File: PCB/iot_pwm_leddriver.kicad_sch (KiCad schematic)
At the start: 17 parts, among them J1 ProgConn-SOICBite, J2 12V PWR, SW1 RESET, SW2 FLASH, U2 ESP-12F

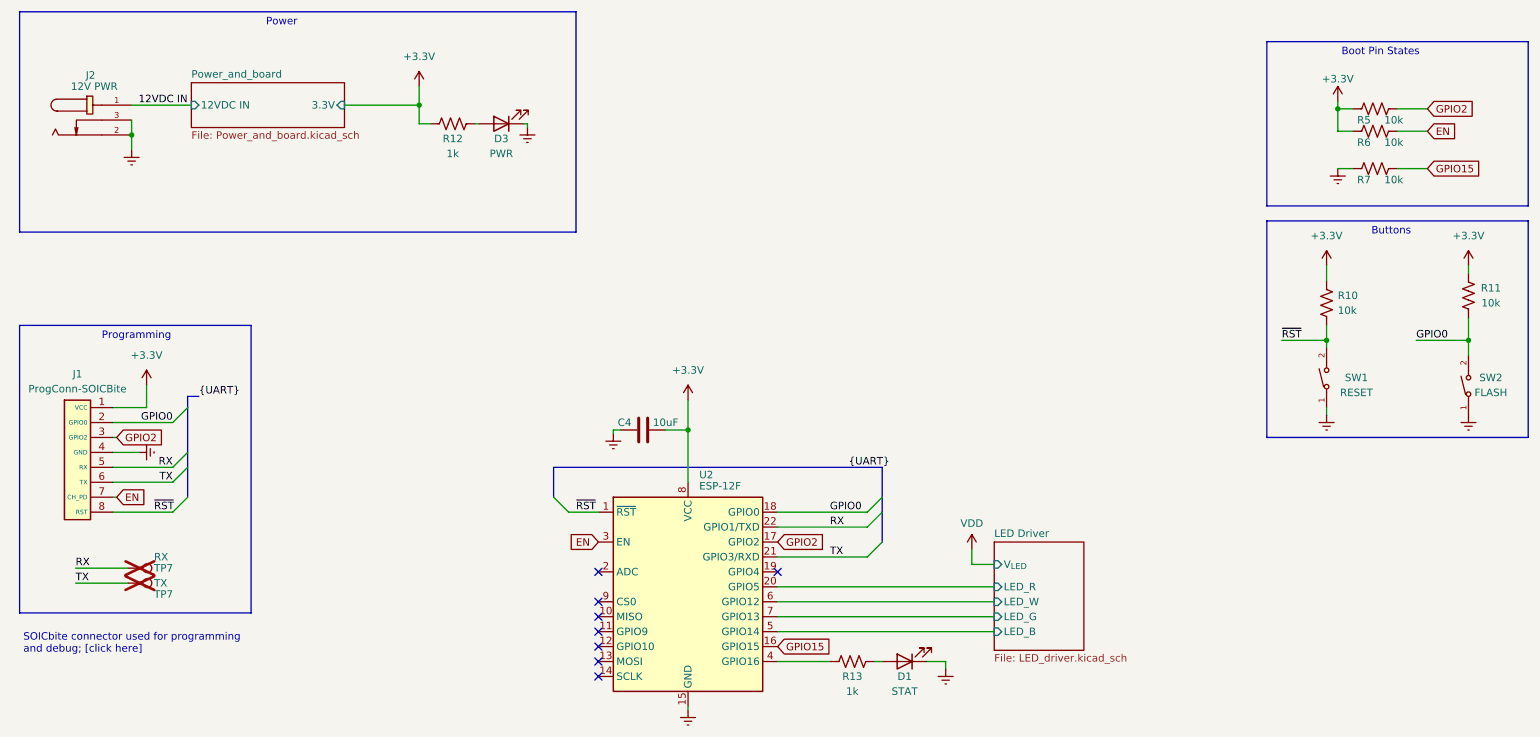
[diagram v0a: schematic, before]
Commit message: schematic and layout cleanup
* plus BOM finalization
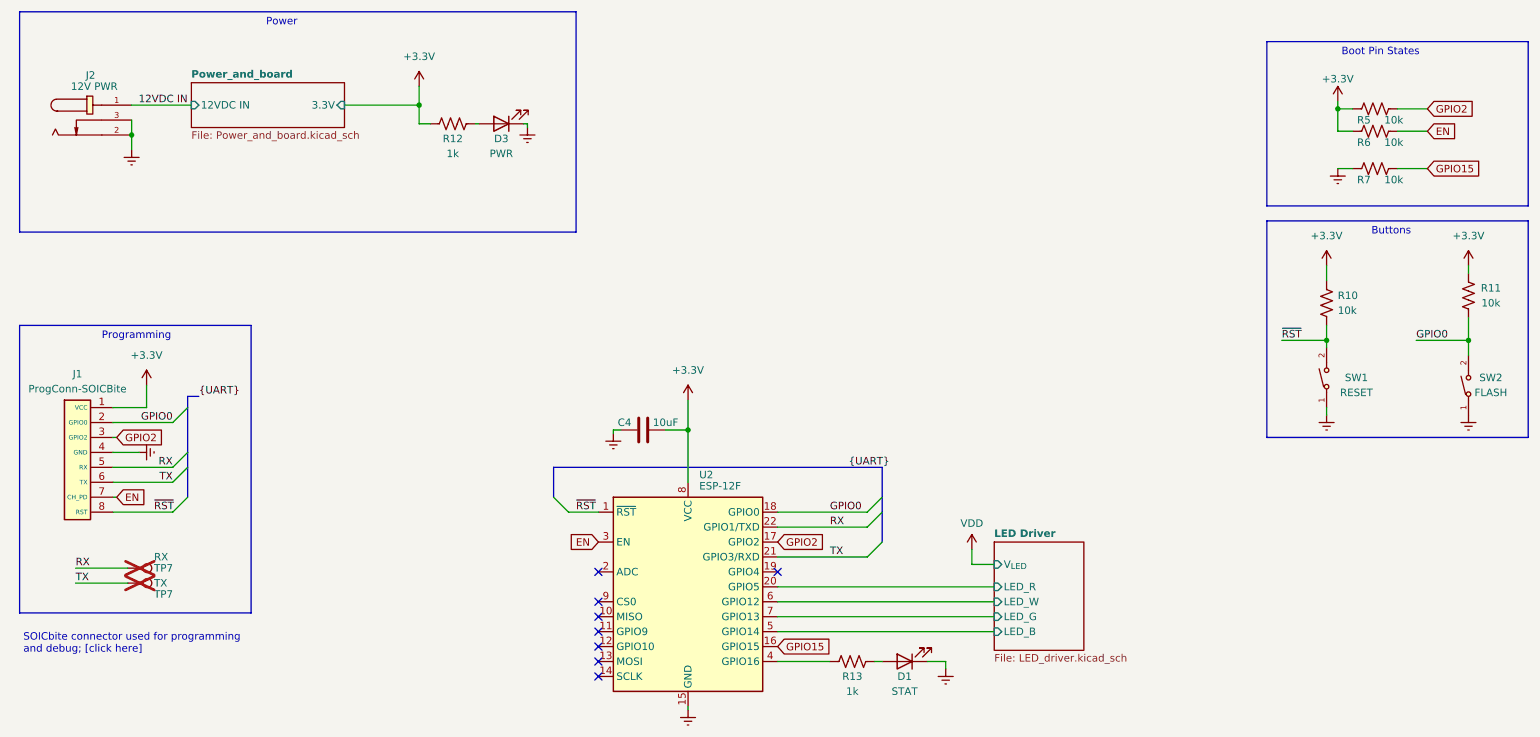
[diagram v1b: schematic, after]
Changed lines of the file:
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@@
     (fill (color 255 229 191 1.0000))
     (property "Sheetname" "LED Driver" (at 185.42 105.3334 0)
-      (effects (font (size 1.27 1.27)) (justify left bottom))
+      (effects (font (size 1.27 1.27) bold) (justify left bottom))
     )
     (property "Sheetfile" "LED_driver.kicad_sch" (at 185.42 125.0446 0)
@@
     (fill (color 255 229 191 1.0000))
     (property "Sheetname" "Power_and_board" (at 48.895 27.2284 0)
-      (effects (font (size 1.27 1.27)) (justify left bottom))
+      (effects (font (size 1.27 1.27) bold) (justify left bottom))
     )
     (property "Sheetfile" "Power_and_board.kicad_sch" (at 48.895 36.1446 0)
